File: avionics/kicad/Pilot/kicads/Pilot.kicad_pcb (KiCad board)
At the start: 6 copper layers, 55 x 35 mm, 111 parts, among them X2Y-CAN 4.7nF X2Y, X2Y-RS485 4.7nF X2Y

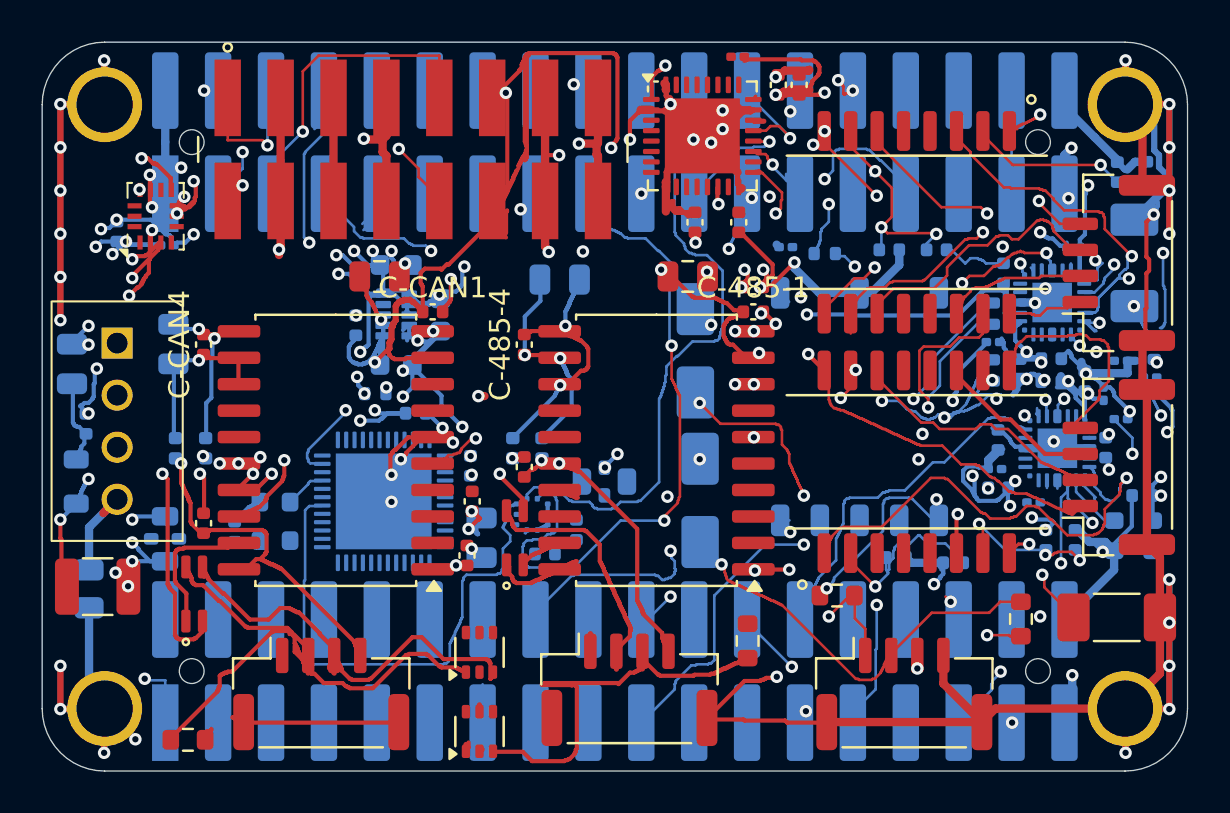
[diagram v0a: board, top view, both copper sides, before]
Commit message: wip(pilot): save in-progress KiCad edits before merge with pilot-gh-tvs
Co-Authored-By: Claude Sonnet 5.5 <noreply@anthropic.com>
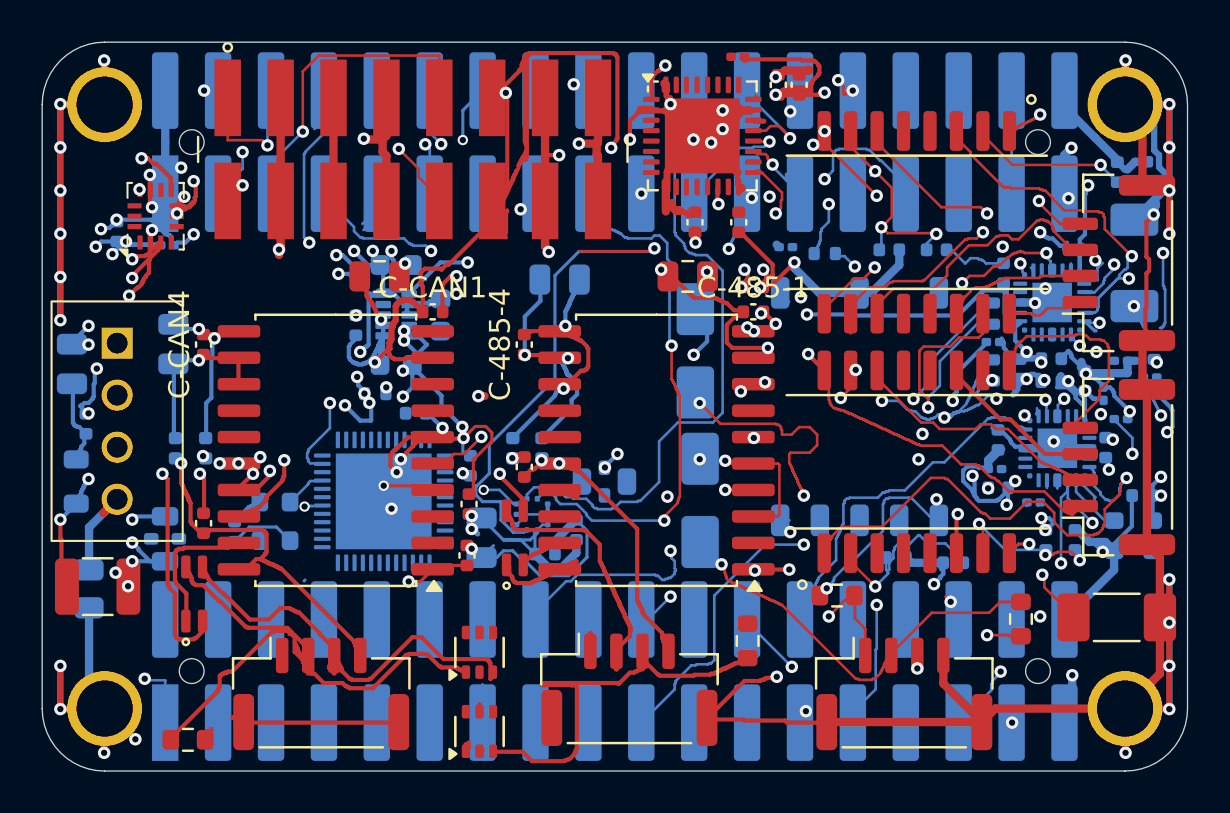
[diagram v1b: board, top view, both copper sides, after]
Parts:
- moved C-1553D 0.20 mm to (141.5, 109.7)
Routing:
- net RS485_DE: track 0.34 -> 33.7 mm, vias 0 -> 2
- net SPI0_CLK: track 4.03 -> 35.7 mm
- net RS485_RX: track 0.00 -> 28.5 mm, vias 0 -> 2
- net CAN_STB: track 0.15 -> 23.5 mm, vias 0 -> 2
- net GND: track 211.2 -> 230.0 mm, vias 72 -> 71
- net +3V3: track 132.9 -> 147.6 mm
- net SPI0_MISO: track 42.6 -> 28.4 mm, vias 3 -> 5
- net ETH_USB1_RXN: track 1.34 -> 9.00 mm, vias 1 -> 2
- net PGND: track 423.9 -> 416.5 mm
- net BARO_INT: track 32.1 -> 26.2 mm
- net +5V: track 150.6 -> 145.2 mm
- net BUS_1553_P: track 21.0 -> 24.0 mm
- net MCAN0_RX: track 18.7 -> 16.2 mm
- net VCC2_RS485_DCDC: track 10.3 -> 11.2 mm
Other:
- copper layers 6 -> 8
